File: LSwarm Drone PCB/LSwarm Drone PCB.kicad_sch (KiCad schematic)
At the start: 0 parts

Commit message: sync
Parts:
- added J1: USB_C_Receptacle, symbol Connector:USB_C_Receptacle
- added U1: RP2350A, Package_DFN_QFN:QFN-60-1EP_7x7mm_P0.4mm_EP3.4x3.4mm, symbol MCU_RaspberryPi:RP2350A
- added U2: ESP32-C3, Package_DFN_QFN:QFN-32-1EP_5x5mm_P0.5mm_EP3.7x3.7mm, symbol MCU_Espressif:ESP32-C3
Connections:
- new net: J1.A1 (GND), J1.A12 (GND), J1.B1 (GND), J1.B12 (GND)
- new net: J1.A4 (VBUS), J1.A9 (VBUS), J1.B4 (VBUS), J1.B9 (VBUS), U1.49 (VREG_VIN)
- new net: U1.1 (IOVDD), U1.11 (IOVDD), U1.20 (IOVDD), U1.30 (IOVDD), U1.38 (IOVDD), U1.45 (IOVDD)
- new net: U1.23 (DVDD), U1.39 (DVDD), U1.6 (DVDD)
- new net: U2.2 (VDD3P3), U2.3 (VDD3P3)
- new net: U2.31 (VDDA), U2.32 (VDDA)

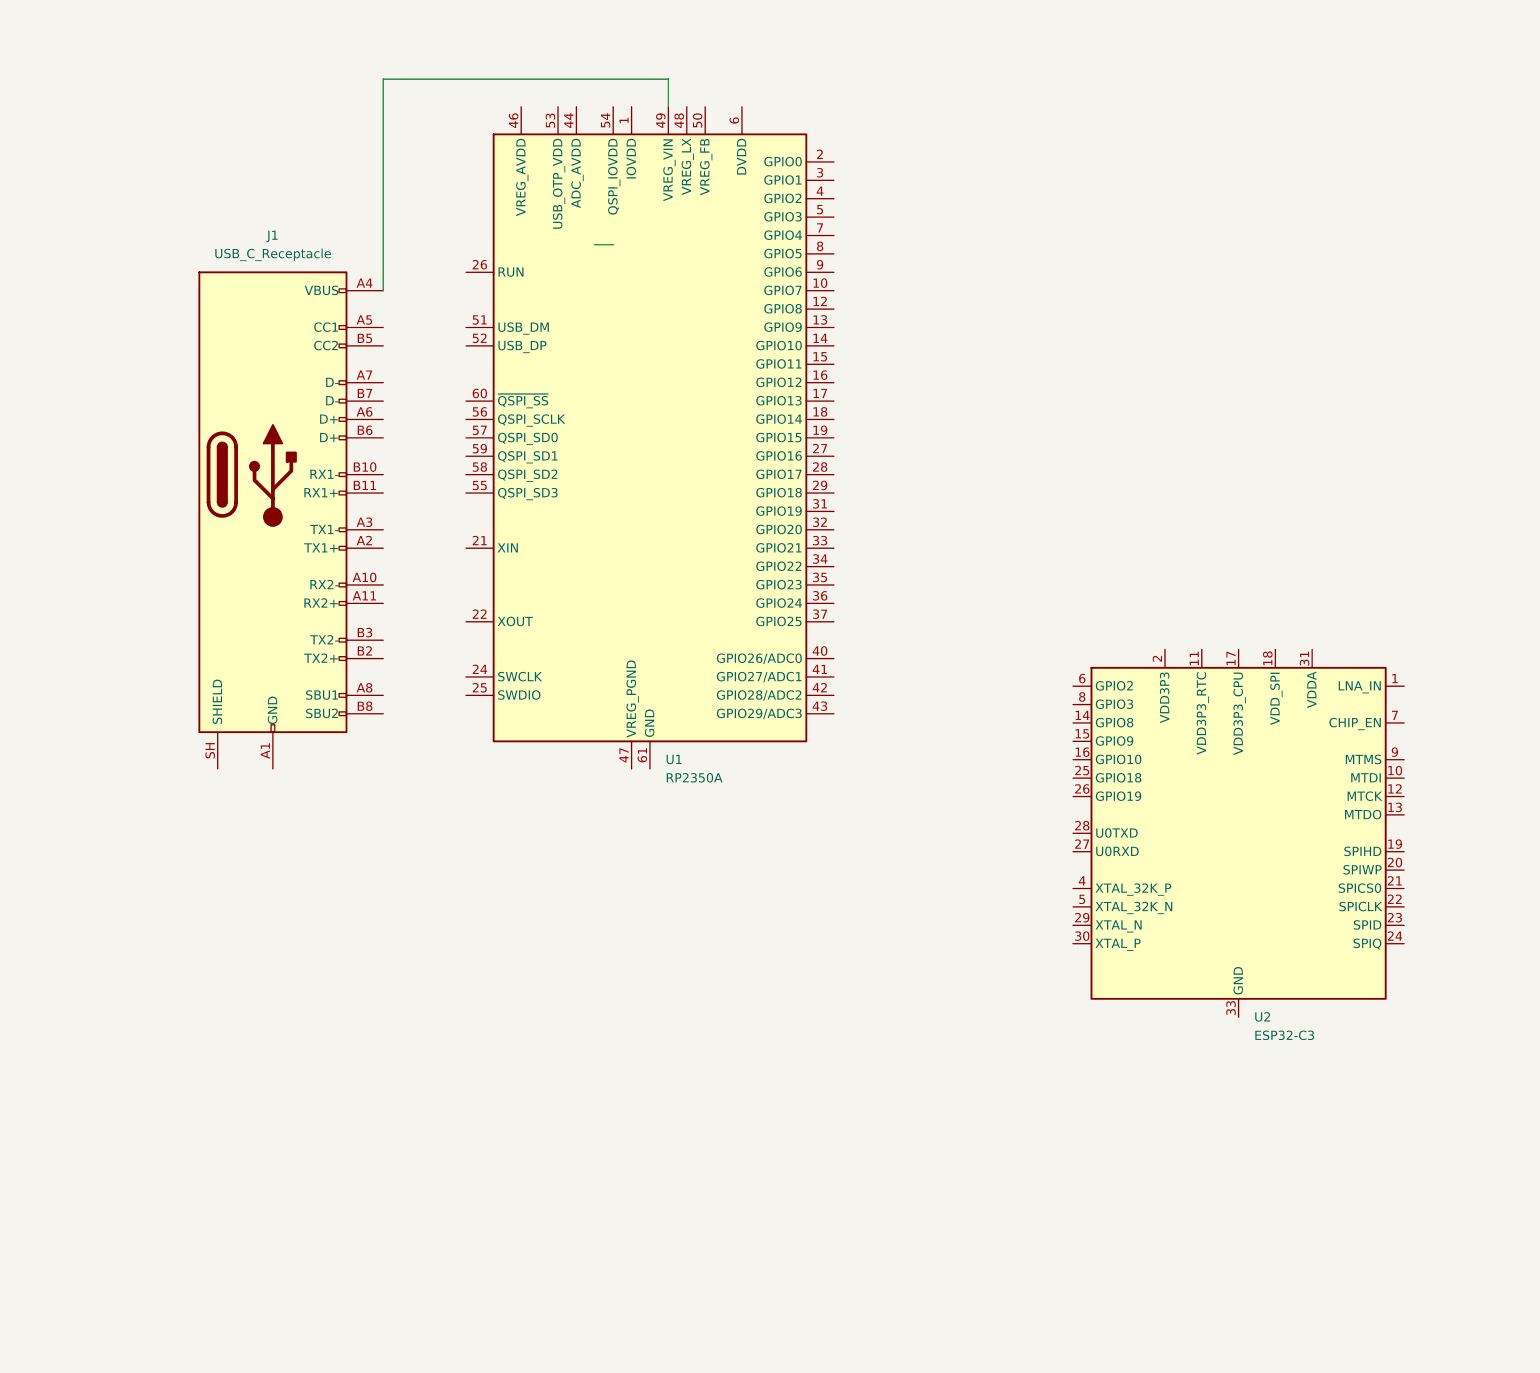
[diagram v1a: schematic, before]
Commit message: sync
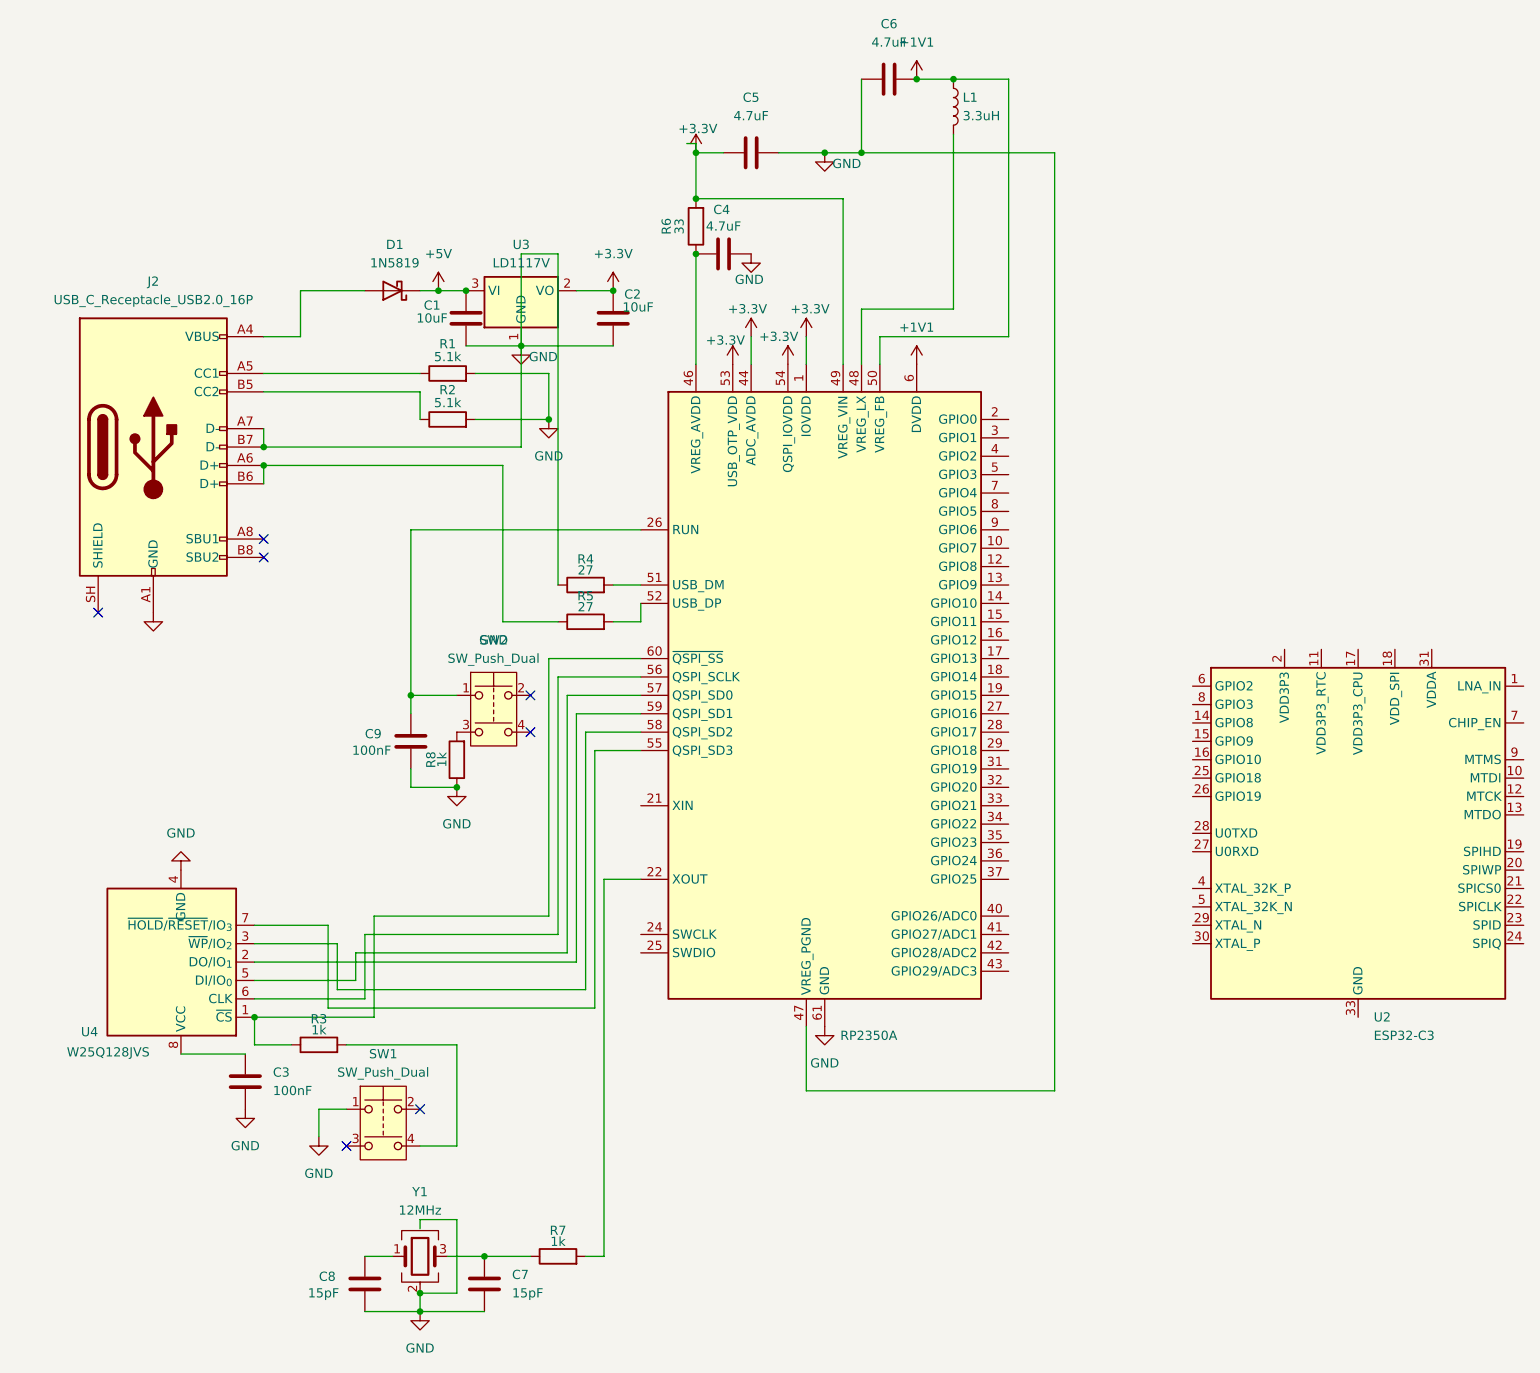
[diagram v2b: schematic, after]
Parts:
- removed J1: USB_C_Receptacle, symbol Connector:USB_C_Receptacle
- added C1, C2: 10uF, symbol Device:C
- added C3, C9: 100nF, symbol Device:C
- added C4, C5, C6: 4.7uF, symbol Device:C
- added C7, C8: 15pF, symbol Device:C
- added D1: 1N5819, Diode_THT:D_DO-41_SOD81_P10.16mm_Horizontal, symbol Diode:1N5819
- added J2: USB_C_Receptacle_USB2.0_16P, symbol Connector:USB_C_Receptacle_USB2.0_16P
- added L1: 3.3uH, symbol Device:L
- added R1, R2: 5.1k, symbol Device:R
- added R3, R7, R8: 1k, symbol Device:R
- added R4, R5: 27, symbol Device:R
- added R6: 33, symbol Device:R
- added SW1, SW2: SW_Push_Dual, symbol Switch:SW_Push_Dual
- added U3: LD1117V, Package_TO_SOT_THT:TO-220-3_Vertical, symbol Regulator_Linear:LD1117V
- added U4: W25Q128JVS, Package_SO:SOIC-8_5.3x5.3mm_P1.27mm, symbol Memory_Flash:W25Q128JVS
- added Y1: 12MHz, symbol Device:Crystal_GND24
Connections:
- net +3.3V: now reaches U1.49 (VREG_VIN)
- net +3.3V: now also U1.1 (IOVDD), U1.11 (IOVDD), U1.20 (IOVDD), U1.30 (IOVDD), U1.38 (IOVDD), U1.44 (ADC_AVDD), U1.45 (IOVDD), U1.53 (USB_OTP_VDD), U1.54 (QSPI_IOVDD), C2.1, C5.1, R6.2, U3.2 (VO)
- net at U1.22 (XOUT): now also R7.2
- net +1V1: now reaches U1.23 (DVDD), U1.39 (DVDD), U1.6 (DVDD)
- net +1V1: now also U1.50 (VREG_FB), C6.2, L1.1
- net at U1.26 (RUN): now also C9.1, SW2.1
- net at U1.46 (VREG_AVDD): now also C4.1, R6.1
- net GND: now reaches U1.47 (VREG_PGND)
- net GND: now also U1.61 (GND), C1.2, C2.2, C3.2, C4.2, C5.2, C6.1, C7.2, C8.2, C9.2, J2.A1 (GND), J2.A12 (GND), J2.A7 (D-), J2.B1 (GND), J2.B12 (GND), J2.B7 (D-), R1.2, R2.2, R4.1, R8.1, SW1.1, U3.1 (GND), U4.4 (GND), Y1.2 (G), Y1.4 (G)
- net at U1.48 (VREG_LX): now also L1.2
- net at U1.51 (USB_DM): now also R4.2
- net at U1.52 (USB_DP): now also R5.2
- net at U1.55 (QSPI_SD3): now also U4.7 (~{HOLD}/~{RESET}/IO_{3})
- net at U1.56 (QSPI_SCLK): now also U4.6 (CLK)
- net at U1.57 (QSPI_SD0): now also U4.5 (DI/IO_{0})
- net at U1.58 (QSPI_SD2): now also U4.3 (~{WP}/IO_{2})
- net at U1.59 (QSPI_SD1): now also U4.2 (DO/IO_{1})
- net at U1.60 (~{QSPI_SS}): now also R3.1, U4.1 (~{CS})
- new net: R8.2, SW2.3
- new net: C7.1, R7.1, Y1.3
- new net: R3.2, SW1.4
- new net: C8.1, Y1.1
- new net: D1.2 (A), J2.A4 (VBUS), J2.A9 (VBUS), J2.B4 (VBUS), J2.B9 (VBUS)
- new net: J2.A5 (CC1), R1.1
- new net: J2.A6 (D+), J2.B6 (D+), R5.1
- new net: J2.B5 (CC2), R2.1
- new net: C3.1, U4.8 (VCC)
- new net +5V: C1.1, D1.1 (K), U3.3 (VI)
- no-connect marks 0 -> 7
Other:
- moved on the sheet: U2
